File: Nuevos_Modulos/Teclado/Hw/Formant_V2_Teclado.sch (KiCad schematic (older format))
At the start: 106 parts

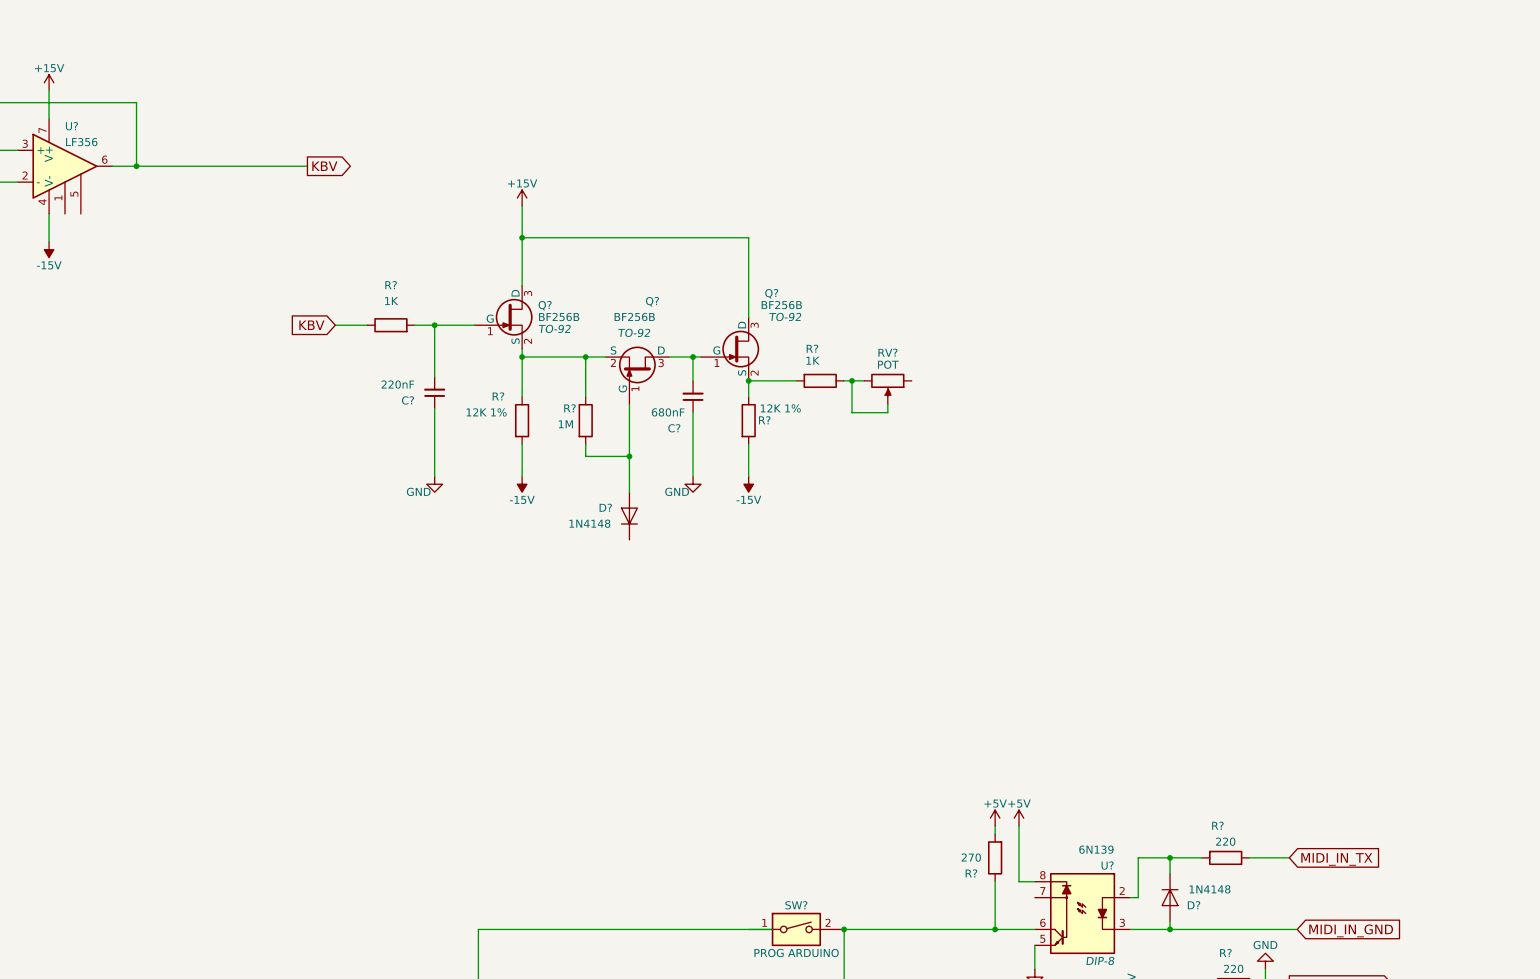
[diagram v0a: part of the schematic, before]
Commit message: Actualizacion HW Teclado
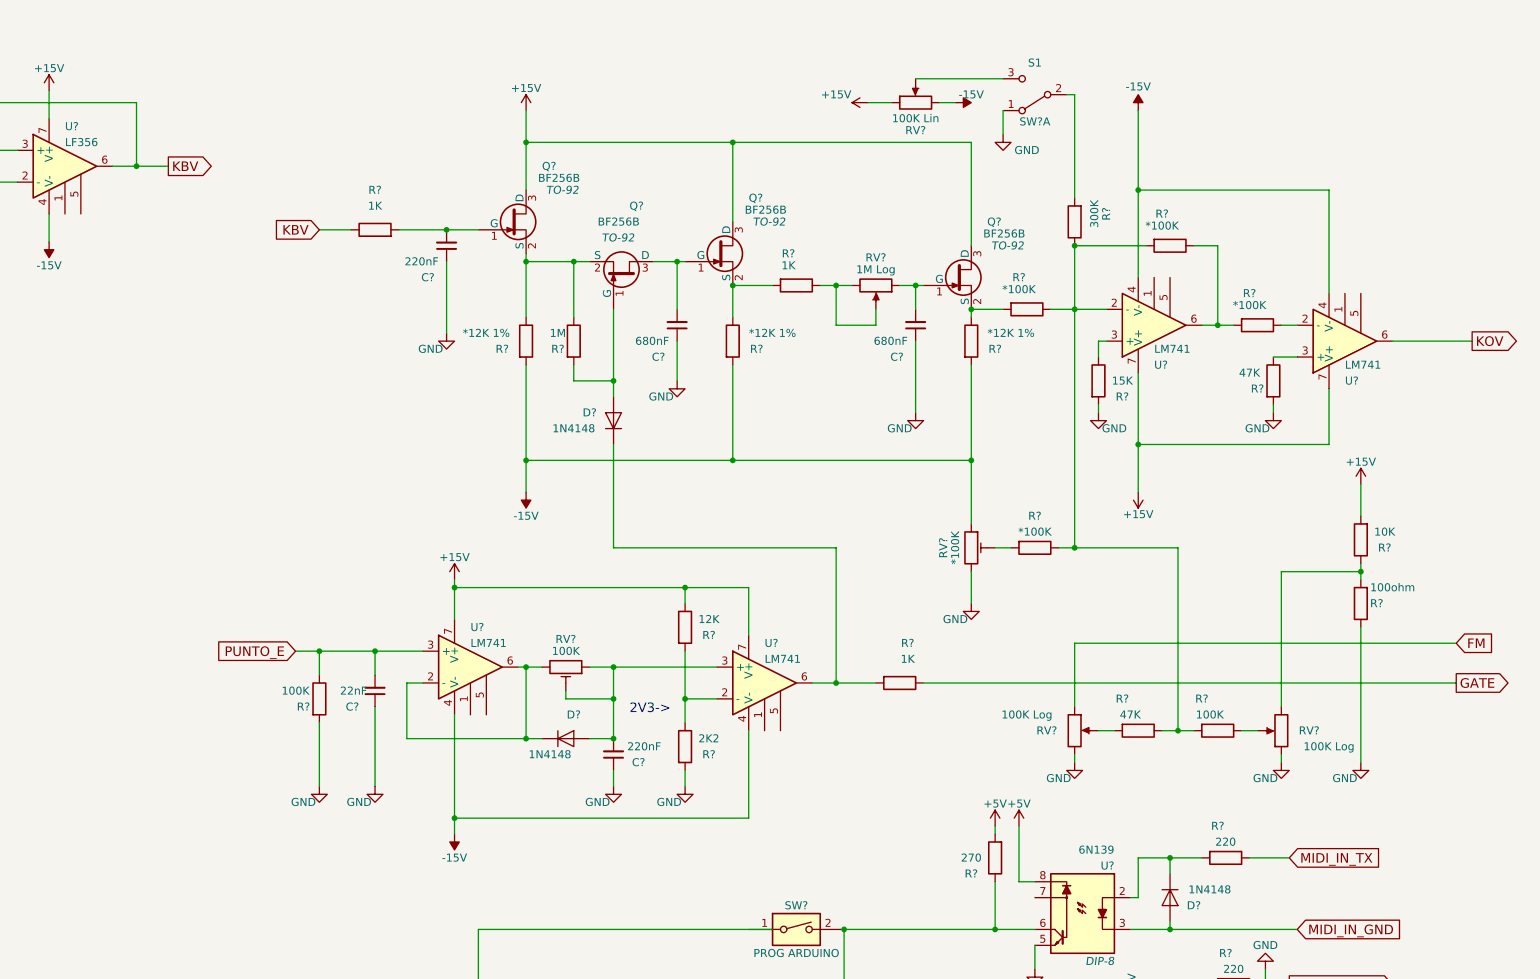
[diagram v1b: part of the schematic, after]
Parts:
- removed C?: 220nF, symbol C_Small
- removed Q?: BF256B, TO-92, symbol BF245B
- removed R?: 12K 1%, symbol R
- removed R?: 1M, symbol R
- removed RV?: POT, symbol POT
- added C?: 680nF, symbol C_Small
- added C? (x2): 220nF, symbol C_Small
- added C?: 22nF, symbol C_Small
- added D?: 1N4148, symbol D
- added Q? (x2): BF256B, TO-92, symbol BF245B
- added R? (x2): *12K 1%, symbol R
- added R? (x4): *100K, symbol R
- added R?: 300K, symbol R
- added R?: 15K, symbol R
- added R? (x2): 47K, symbol R
- added R?: 1M, symbol R
- added R? (x2): 100K, symbol R
- added R?: 12K, symbol R
- added R?: 2K2, symbol R
- added R?: 1K, symbol R
- added R?: 10K, symbol R
- added R?: 100ohm, symbol R
- added RV?: 1M Log, symbol POT
- added RV?: 100K Lin, symbol POT
- added RV?: 100K, symbol POT_TRIM
- added RV?: *100K, symbol POT_TRIM
- added RV? (x2): 100K Log, symbol POT
- added SW?: S1, symbol SW_DPDT_x2
- added U? (x4): LM741, symbol LM741
- R?: value 12K 1% -> *12K 1%
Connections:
- net +15V: now also Q?.3 (D), Q?.3 (D), R?.1, R?.2, RV?.1, U?.7 (V+), U?.7 (V+), U?.7 (V+), U?.7 (V+)
- net -15V: now also R?.2, R?.2, RV?.1, RV?.3, U?.4 (V-), U?.4 (V-), U?.4 (V-), U?.4 (V-)
- net GND: now also C?.1, C?.1, C?.1, C?.1, R?.1, R?.2, R?.2, R?.2, R?.2, RV?.1, RV?.3, RV?.3, SW?.1 (A)
- net PUNTO_E: now also C?.2, R?.1, U?.3 (+)
- net at R?.2: now also C?.2, Q?.1 (G)
- net at Q?.2 (S): now also Q?.2 (S), R?.1, R?.1
- net at D?.2 (A), Q?.1 (G): now also R?.2
- net at D?.1 (K): now also R?.2, U?.6
- net at R?.1: now also RV?.2, RV?.3
- new net: C?.2, Q?.1 (G), RV?.1
- new net: Q?.2 (S), R?.1, R?.2
- new net: R?.1, R?.1, R?.1, R?.1, R?.2, R?.2, U?.2 (-)
- new net: R?.2, SW?.2 (B)
- new net: R?.1, U?.3 (+) (x2)
- new net: R?.1, R?.2, U?.6
- new net: R?.1, U?.2 (-)
- new net: RV?.2, SW?.3 (C)
- new net: D?.1 (K), RV?.3, U?.2 (-), U?.6
- new net: C?.2, D?.2 (A), RV?.1, RV?.2, U?.3 (+)
- new net: R?.1, R?.2, U?.2 (-)
- new net: R?.2, RV?.2 (x2)
- new net: R?.1, RV?.2
- new net: R?.1, R?.2, RV?.3
- new net FM: RV?.1
- new net GATE: R?.1
- new net KOV: U?.6
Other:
- note added: "2V3->"
- moved on the sheet: C?, D?, Q?, R?
